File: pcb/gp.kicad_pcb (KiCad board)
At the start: 2 copper layers, 52.1 x 20.3 mm, 31 parts, among them J1 USB-C, SW1 TS-1088R-02526, SW2 TS-1088R-02526, U1 XC6206P332MR, U2 STM32F103CBT6, U3 W25Q32JVSS, Y1 16Mhz

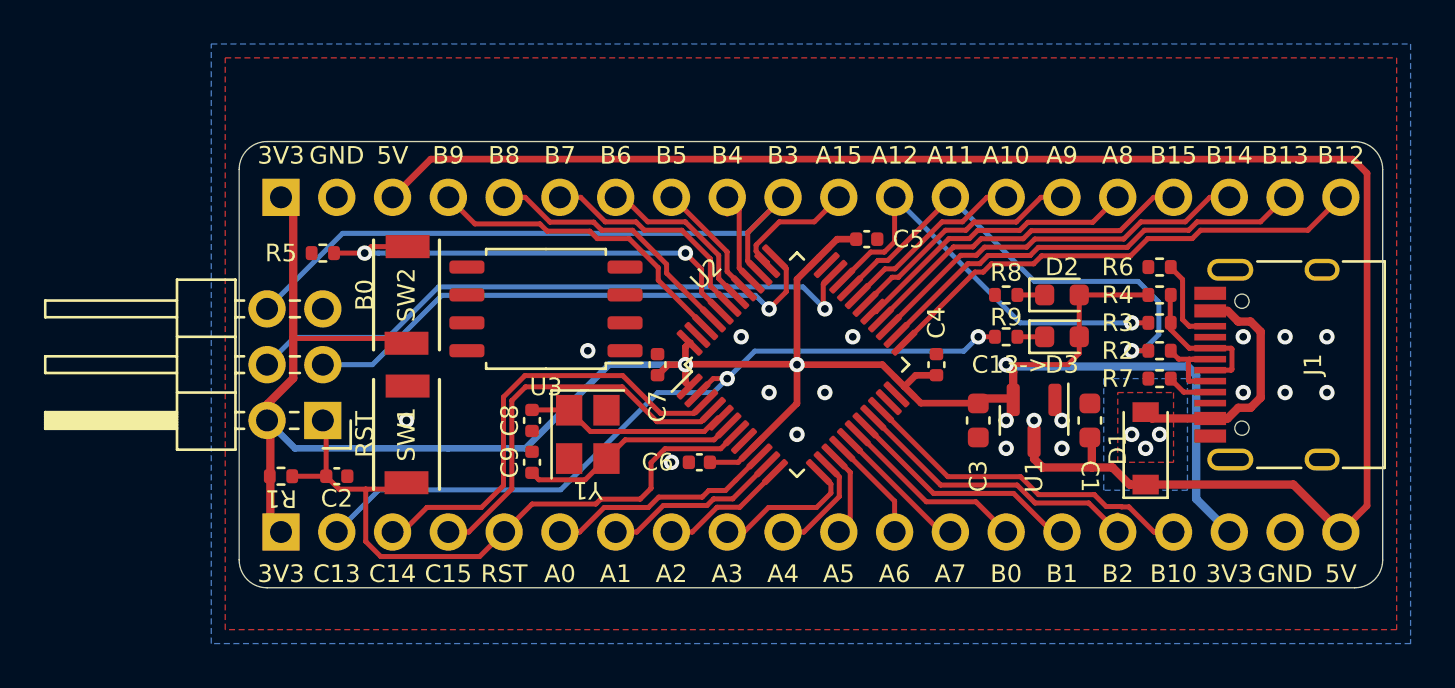
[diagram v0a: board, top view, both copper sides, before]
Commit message: Hmmmm
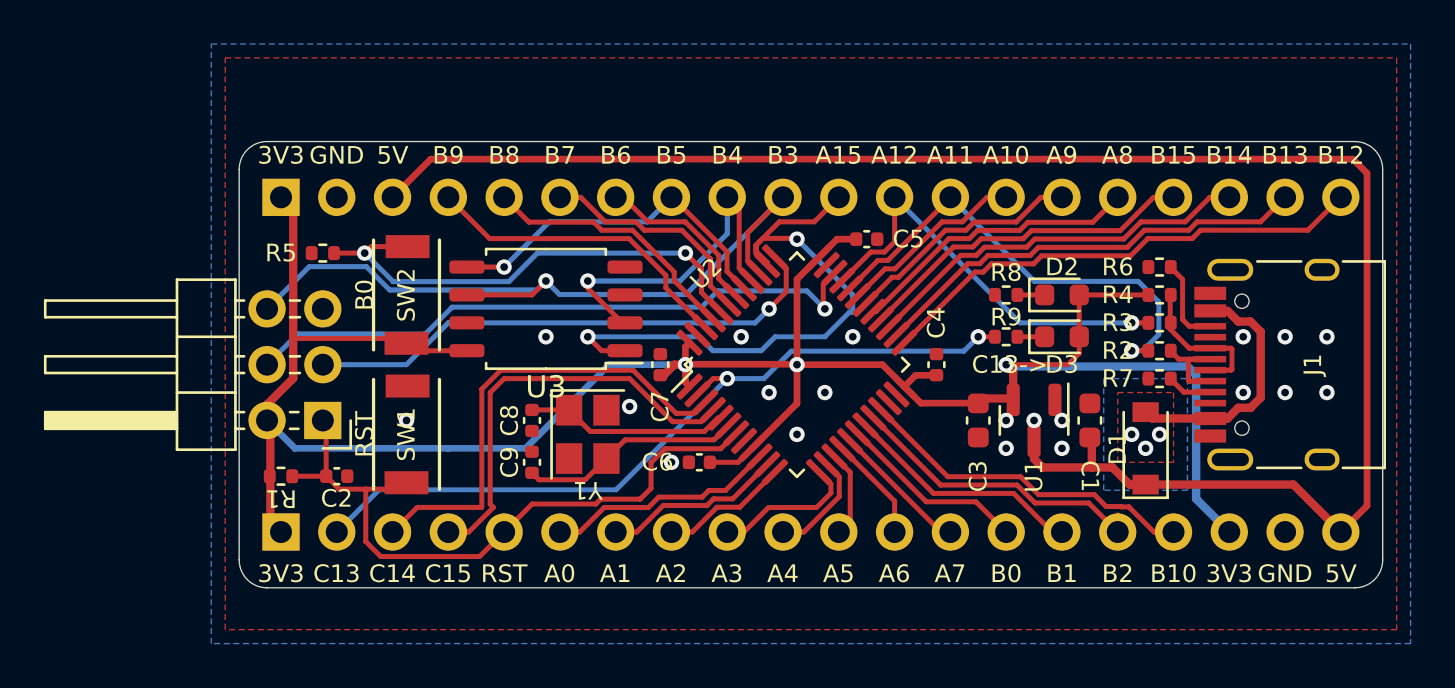
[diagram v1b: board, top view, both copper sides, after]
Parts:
- moved C7 0.13 mm to (170.9, 101.6)
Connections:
- J1 pad A8: Net-(J1-PadA8) -> unconnected-(J1-PadA8)
- J1 pad B8: Net-(J1-PadB8) -> unconnected-(J1-PadB8)
- U2 pad 22: Net-(U2-Pad22) -> unconnected-(U2-Pad22)
- U3 pad 3: Net-(U3-Pad3) -> unconnected-(U3-Pad3)
- U3 pad 7: Net-(U3-Pad7) -> unconnected-(U3-Pad7)
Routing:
- net A15: track 6.63 -> 29.1 mm, vias 0 -> 2
- net B4: track 5.03 -> 16.6 mm, vias 0 -> 1
- net B5: track 6.23 -> 16.9 mm, vias 0 -> 1
- net B3: track 30.6 -> 35.8 mm, vias 0 -> 1
- net +3V3: track 105.5 -> 108.3 mm
- net C15: track 18.0 -> 19.2 mm
- net BO0: track 21.4 -> 22.5 mm
- net C14: track 20.5 -> 21.5 mm
- net SWCLK: track 24.8 -> 24.3 mm
- net GND: vias 17 -> 18

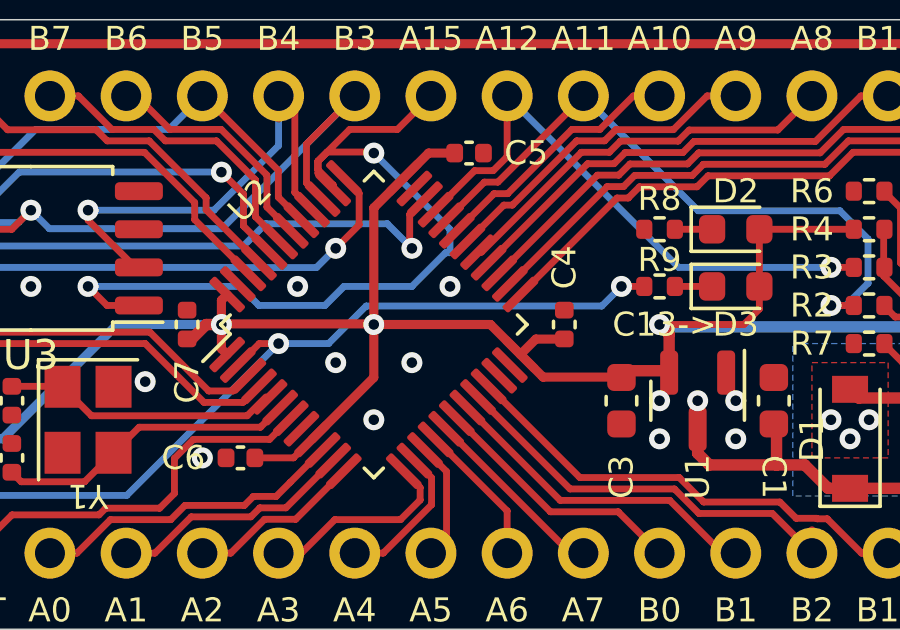
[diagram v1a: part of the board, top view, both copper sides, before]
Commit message: Tweaking
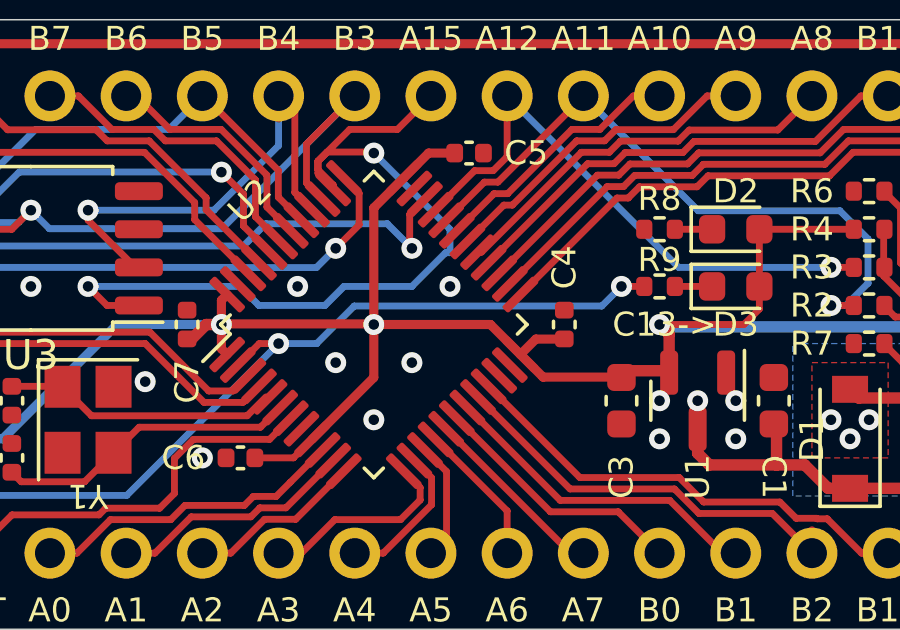
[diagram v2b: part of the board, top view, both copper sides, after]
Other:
- rule pad_to_mask_clearance: 0.05 -> 0

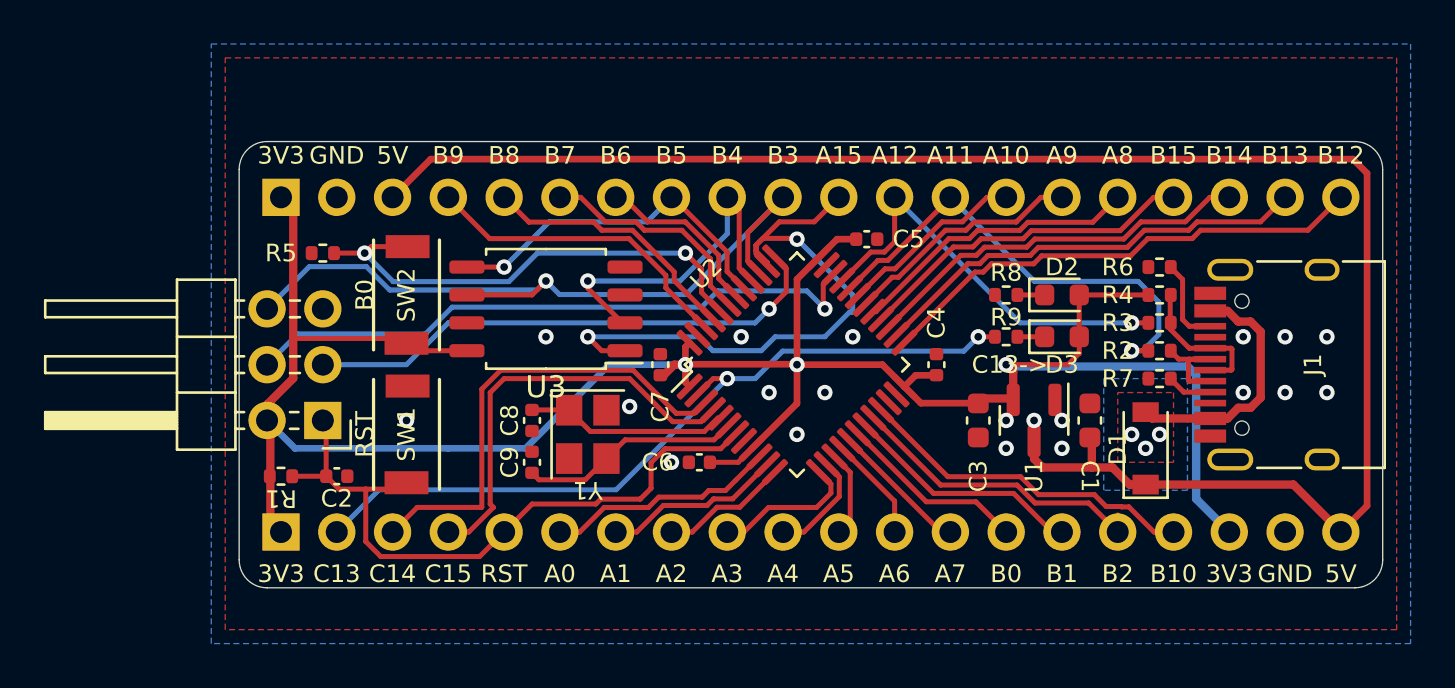
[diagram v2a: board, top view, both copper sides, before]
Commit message: Hmmmm
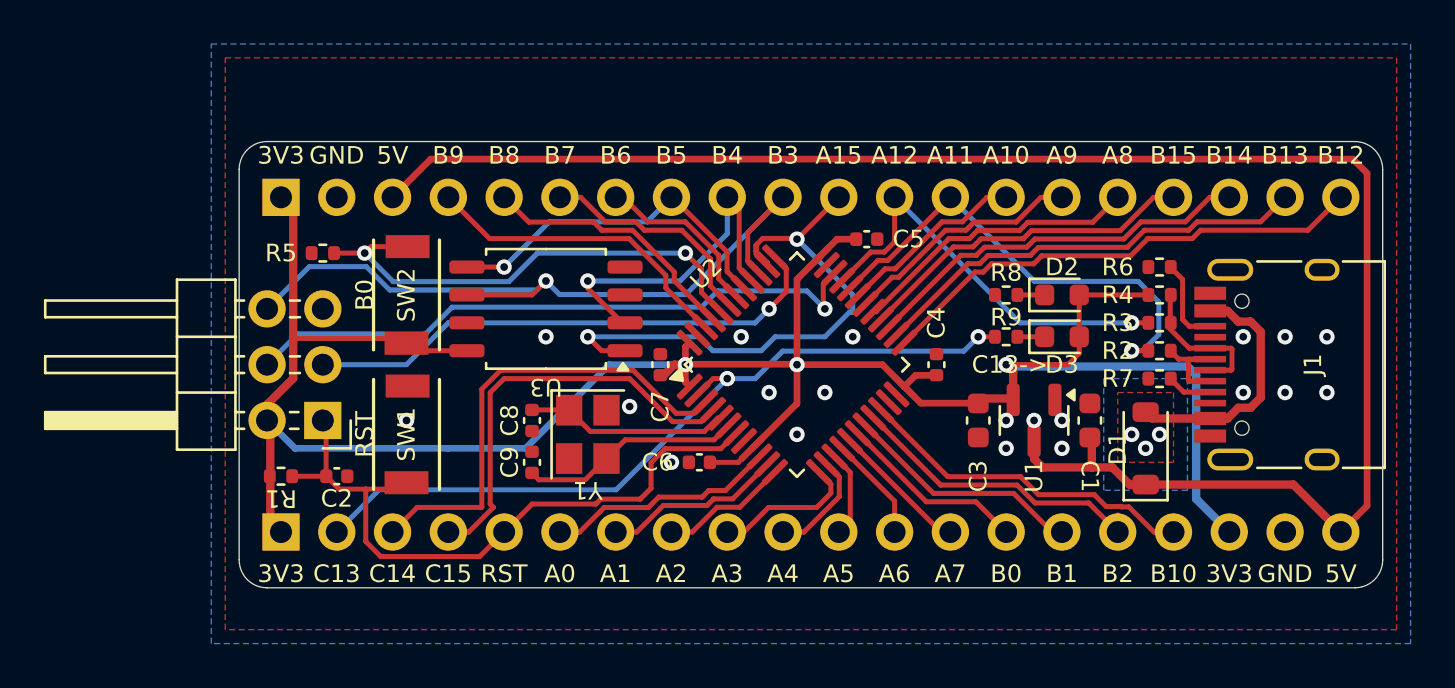
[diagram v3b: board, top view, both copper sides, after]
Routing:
- net A15: track 29.1 -> 26.3 mm
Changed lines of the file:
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@@
         (effects (font (size 1 1) (thickness 0.15)))
     )
-    (fp_line (start 0 -1.56) (end -1.675 -1.56)
+    (fp_line (start 0 -1.56) (end -0.65 -1.56)
       (stroke (width 0.12) (type solid)) (layer "F.SilkS"))
     (fp_line (start 0 -1.56) (end 0.65 -1.56)
@@
     (fp_line (start 0 1.56) (end 0.65 1.56)
       (stroke (width 0.12) (type solid)) (layer "F.SilkS"))
+    (fp_poly
+      (pts
+        (xy -1.1625 -1.51)
+        (xy -1.4025 -1.84)
+        (xy -0.9225 -1.84)
+        (xy -1.1625 -1.51)
+      )
+      (stroke (width 0.12) (type solid)) (fill solid) (layer "F.SilkS"))
     (fp_line (start -1.92 -1.7) (end -1.92 1.7)
       (stroke (width 0.05) (type solid)) (layer "F.CrtYd"))
@@
     (pad "3" smd roundrect (at 0.9375 0 270) (size 1.475 0.6) (layers "F.Cu" "F.Paste" "F.Mask") (roundrect_rratio 0.25)
       (net 45 "+5V") (pinfunction "VI") (pintype "power_in"))
-    (model "${KICAD6_3DMODEL_DIR}/Package_TO_SOT_SMD.3dshapes/SOT-23.wrl"
+    (model "${KICAD7_3DMODEL_DIR}/Package_TO_SOT_SMD.3dshapes/SOT-23.wrl"
       (offset (xyz 0 0 0))
       (scale (xyz 1 1 1))
@@
         (effects (font (size 1 1) (thickness 0.15)))
     )
-    (fp_line (start -2.25 -1) (end -2.25 1)
-      (stroke (width 0.12) (type solid)) (layer "F.SilkS"))
-    (fp_line (start -2.25 -1) (end 1.65 -1)
-      (stroke (width 0.12) (type solid)) (layer "F.SilkS"))
-    (fp_line (start -2.25 1) (end 1.65 1)
+    (fp_line (start -2.36 -1) (end -2.36 1)
+      (stroke (width 0.12) (type solid)) (layer "F.SilkS"))
+    (fp_line (start -2.36 -1) (end 1.65 -1)
+      (stroke (width 0.12) (type solid)) (layer "F.SilkS"))
+    (fp_line (start -2.36 1) (end 1.65 1)
       (stroke (width 0.12) (type solid)) (layer "F.SilkS"))
     (fp_line (start -2.35 -1.15) (end -2.35 1.15)
@@
     (fp_line (start 1.4 0.9) (end -1.4 0.9)
       (stroke (width 0.1) (type solid)) (layer "F.Fab"))
-    (pad "1" smd rect (at -1.65 0 90) (size 0.9 1.2) (layers "F.Cu" "F.Paste" "F.Mask")
+    (pad "1" smd roundrect (at -1.65 0 90) (size 0.9 1.2) (layers "F.Cu" "F.Paste" "F.Mask") (roundrect_rratio 0.25)
       (net 45 "+5V") (pinfunction "K") (pintype "passive"))
-    (pad "2" smd rect (at 1.65 0 90) (size 0.9 1.2) (layers "F.Cu" "F.Paste" "F.Mask")
+    (pad "2" smd roundrect (at 1.65 0 90) (size 0.9 1.2) (layers "F.Cu" "F.Paste" "F.Mask") (roundrect_rratio 0.25)
       (net 2 "VBUS") (pinfunction "A") (pintype "passive"))
     (model "${KICAD6_3DMODEL_DIR}/Diode_SMD.3dshapes/D_SOD-123.wrl"
@@
     (fp_line (start -3.61 -3.61) (end -3.61 -3.16)
       (stroke (width 0.12) (type solid)) (layer "F.SilkS"))
-    (fp_line (start -3.61 -3.16) (end -4.9 -3.16)
-      (stroke (width 0.12) (type solid)) (layer "F.SilkS"))
     (fp_line (start -3.61 3.61) (end -3.61 3.16)
       (stroke (width 0.12) (type solid)) (layer "F.SilkS"))
@@
     (fp_line (start 3.61 3.61) (end 3.61 3.16)
       (stroke (width 0.12) (type solid)) (layer "F.SilkS"))
+    (fp_poly
+      (pts
+        (xy -4.2 -3.16)
+        (xy -4.54 -3.63)
+        (xy -3.86 -3.63)
+        (xy -4.2 -3.16)
+      )
+      (stroke (width 0.12) (type solid)) (fill solid) (layer "F.SilkS"))
     (fp_line (start -5.15 -3.15) (end -5.15 0)
       (stroke (width 0.05) (type solid)) (layer "F.CrtYd"))
@@
     (pad "48" smd roundrect (at -2.75 -4.1625 45) (size 0.3 1.475) (layers "F.Cu" "F.Paste" "F.Mask") (roundrect_rratio 0.25)
       (net 3 "+3V3") (pinfunction "VDD") (pintype "power_in"))
-    (model "${KICAD6_3DMODEL_DIR}/Package_QFP.3dshapes/LQFP-48_7x7mm_P0.5mm.wrl"
+    (model "${KICAD7_3DMODEL_DIR}/Package_QFP.3dshapes/LQFP-48_7x7mm_P0.5mm.wrl"
       (offset (xyz 0 0 0))
       (scale (xyz 1 1 1))
@@
     (property "ki_keywords" "flash memory SPI")
     (attr smd)
-    (fp_text reference "U3" (at 0 -3.56 180) (layer "F.SilkS")
-        (effects (font (size 1 1) (thickness 0.15)))
+    (fp_text reference "U3" (at 0 -3.56 180 unlocked) (layer "F.SilkS")
+        (effects (font (size 0.8 0.8) (thickness 0.15)))
     )
     (fp_text value "W25Q32JVSS" (at 0 3.56 180) (layer "F.Fab")
@@
     (fp_line (start -2.725 -2.725) (end -2.725 -2.465)
       (stroke (width 0.12) (type solid)) (layer "F.SilkS"))
-    (fp_line (start -2.725 -2.465) (end -4.4 -2.465)
-      (stroke (width 0.12) (type solid)) (layer "F.SilkS"))
     (fp_line (start -2.725 2.725) (end -2.725 2.465)
       (stroke (width 0.12) (type solid)) (layer "F.SilkS"))
@@
     (fp_line (start 2.725 2.725) (end 2.725 2.465)
       (stroke (width 0.12) (type solid)) (layer "F.SilkS"))
+    (fp_poly
+      (pts
+        (xy -3.5075 -2.465)
+        (xy -3.7475 -2.795)
+        (xy -3.2675 -2.795)
+        (xy -3.5075 -2.465)
+      )
+      (stroke (width 0.12) (type solid)) (fill solid) (layer "F.SilkS"))
     (fp_line (start -4.65 -2.86) (end -4.65 2.86)
       (stroke (width 0.05) (type solid)) (layer "F.CrtYd"))
@@
     (pad "8" smd roundrect (at 3.6 -1.905 180) (size 1.6 0.6) (layers "F.Cu" "F.Paste" "F.Mask") (roundrect_rratio 0.25)
       (net 3 "+3V3") (pinfunction "VCC") (pintype "power_in"))
-    (model "${KICAD6_3DMODEL_DIR}/Package_SO.3dshapes/SO-8_5.3x6.2mm_P1.27mm.wrl"
+    (model "${KICAD7_3DMODEL_DIR}/Package_SO.3dshapes/SOIC-8_5.23x5.23mm_P1.27mm.wrl"
       (offset (xyz 0 0 0))
       (scale (xyz 1 1 1))
@@
   (segment (start 158.621864 98.2) (end 157.558075 97.136211) (width 0.2286) (layer "B.Cu") (net 13))
   (segment (start 175.812658 97.065678) (end 175.812658 96.947888) (width 0.2286) (layer "F.Cu") (net 14))
-  (segment (start 177.953299 95.096701) (end 179.07 93.98) (width 0.2286) (layer "F.Cu") (net 14))
-  (segment (start 175.303011 96.155155) (end 176.361465 95.096701) (width 0.2286) (layer "F.Cu") (net 14))
-  (segment (start 176.361465 95.096701) (end 177.953299 95.096701) (width 0.2286) (layer "F.Cu") (net 14))
+  (segment (start 177.165 95.885) (end 179.07 93.98) (width 0.2286) (layer "F.Cu") (net 14))
   (segment (start 175.812658 97.065678) (end 175.303502 96.556522) (width 0.2286) (layer "F.Cu") (net 14))
   (segment (start 177.129414 95.849414) (end 177.165 95.885) (width 0.2286) (layer "F.Cu") (net 14))
   (segment (start 168.275 100.965) (end 169.335 100.965) (width 0.2286) (layer "F.Cu") (net 14))
   (segment (start 175.303502 96.15536) (end 175.609448 95.849414) (width 0.2286) (layer "F.Cu") (net 14))
-  (segment (start 178.478011 94.571989) (end 179.07 93.98) (width 0.2286) (layer "F.Cu") (net 14))
   (segment (start 175.812658 96.947888) (end 175.303011 96.438241) (width 0.2286) (layer "F.Cu") (net 14))
   (segment (start 168.275 100.965) (end 167.64 100.33) (width 0.2286) (layer "F.Cu") (net 14))
